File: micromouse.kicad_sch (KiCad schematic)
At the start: 12 parts, among them SW1 SW_SPST, SW2 SW_Push, U1 BUCK, U2 STM32 Blackpill, U3 N20 encoder right, U4 N20 encoder left, U5 TB6612FNG, U6 VL53L0X left, U7 VL53L0X right, U8 VL53L0X middle

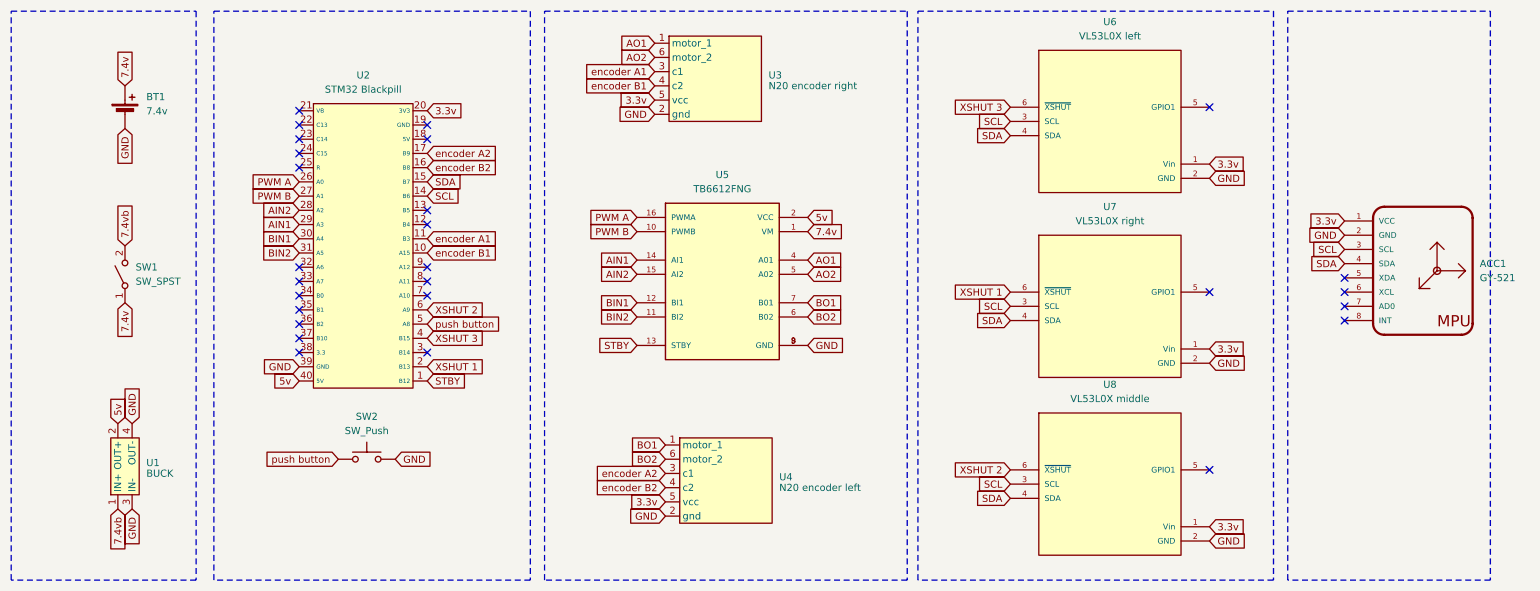
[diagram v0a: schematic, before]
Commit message: schematic and footprint changes
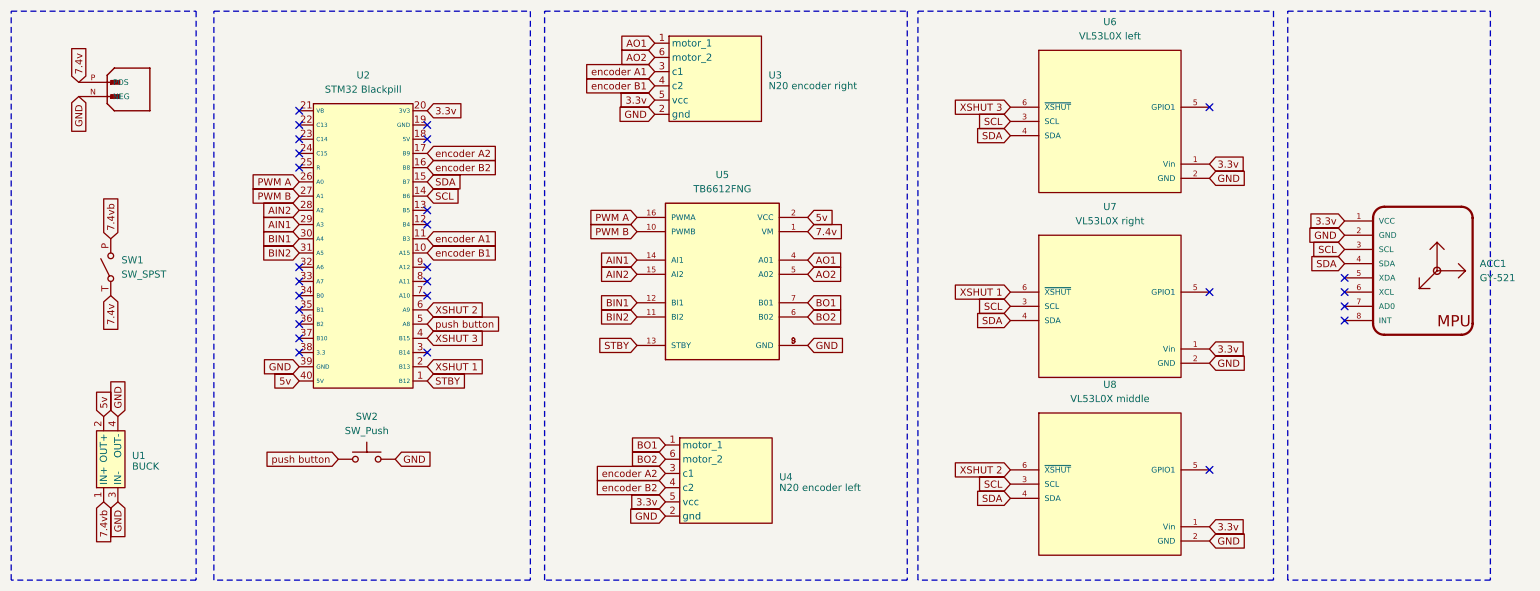
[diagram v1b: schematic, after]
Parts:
- removed BT1: 7.4v, symbol Device:Battery_Cell
- removed U5: TB6612FNG, TB6612FNG:TB6612FNG, symbol tb6612fng:ROB-14450
- added J1: XT60-M, XT60:AMASS_XT60-M, symbol XT60-M:XT60-M
- added U5: TB6612FNG, TB6612FNG:TB6612FNG, symbol TB66:TB6612FNG
- U3, U4: footprint Connector_PinHeader_2.00mm:PinHeader_1x06_P2.00mm_Vertical -> Connector_PinHeader_2.54mm:PinHeader_1x06_P2.54mm_Vertical
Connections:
- net 5v: now also U5.2 (VCC)
- net 7.4v: now also SW1.T (A), J1.P (POS), U5.1 (VM); no longer SW1.1 (A)
- net 7.4vb: now also SW1.P (B); no longer SW1.2 (B)
- net AIN1: now also U5.14 (AI1)
- net AIN2: now also U5.15 (AI2)
- net AO1 : now also U5.4 (A01)
- net AO2: now also U5.5 (A02)
- net BIN1: now also U5.12 (BI1)
- net BIN2: now also U5.11 (BI2)
- net BO1: now also U5.7 (B01)
- net BO2: now also U5.6 (B02)
- net GND: now also J1.N (NEG), U5.3 (GND), U5.8 (GND), U5.9 (GND)
- net PWM A: now also U5.16 (PWMA)
- net PWM B: now also U5.10 (PWMB)
- net STBY: now also U5.13 (STBY)
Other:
- moved on the sheet: SW1, U1

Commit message: routing
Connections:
- net AO1  is gone; now on net AO1: U5.4 (A01)
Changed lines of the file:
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@@
 		)
 	)
-	(global_label "AO1 "
+	(global_label "AO1"
 		(shape input)
 		(at 158.115 84.455 0)
@@
 		)
 		(property "Intersheetrefs" "${INTERSHEET_REFS}"
-			(at 165.6964 84.455 0)
+			(at 164.7288 84.455 0)
 			(effects
 				(font

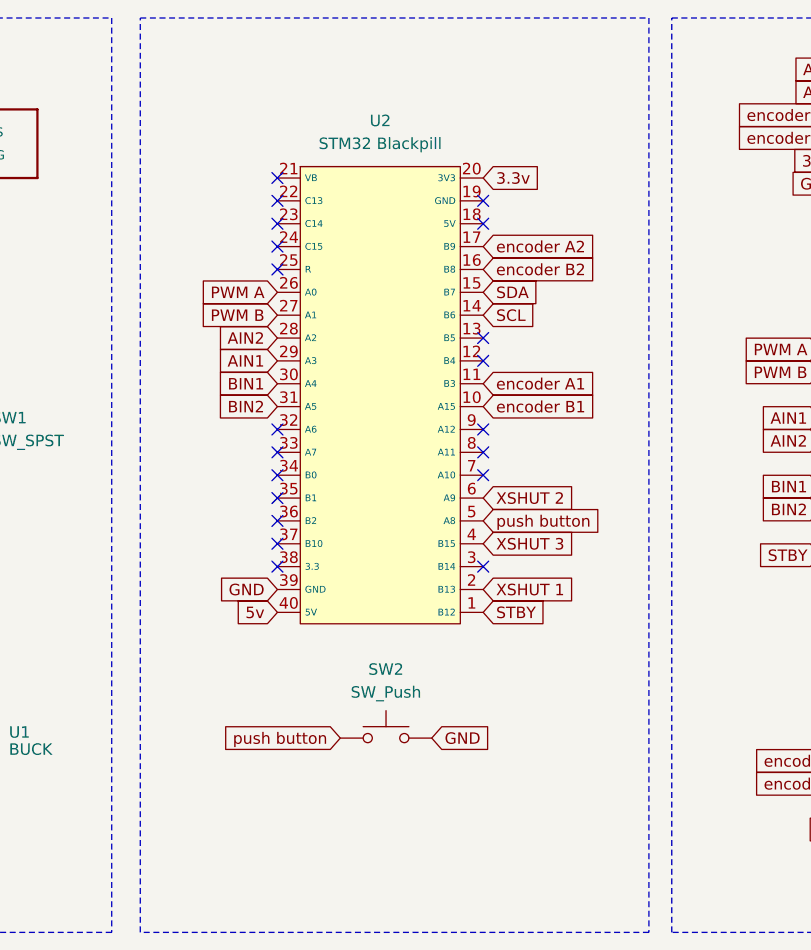
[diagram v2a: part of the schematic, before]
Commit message: ll
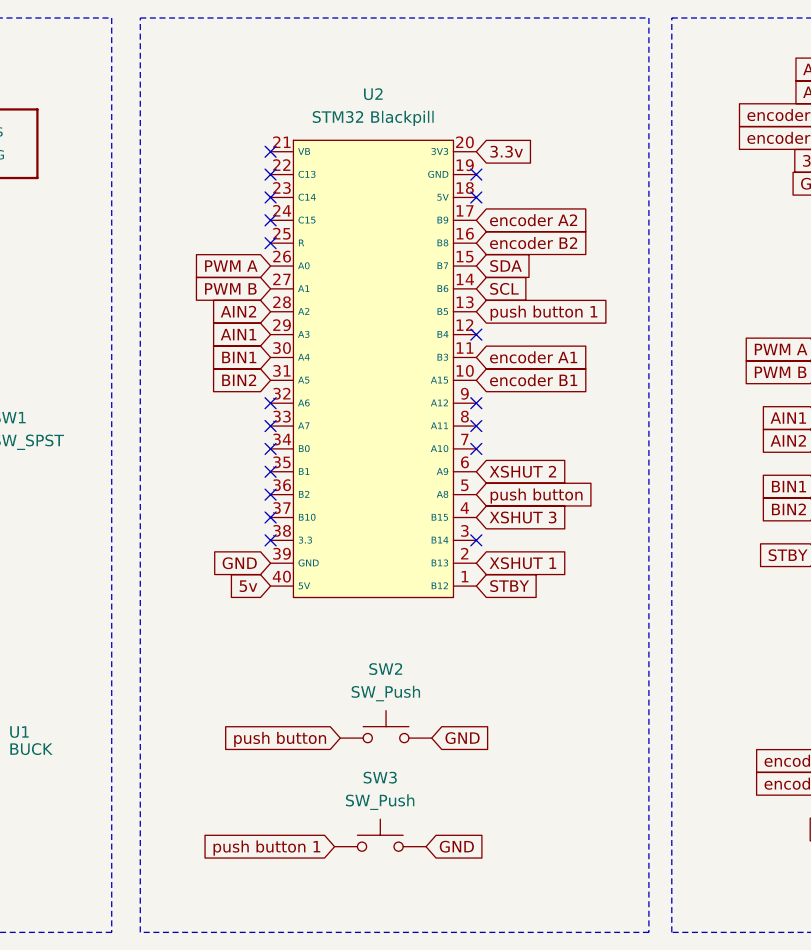
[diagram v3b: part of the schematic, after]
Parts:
- added SW3: SW_Push, push button:push_button, symbol Switch:SW_Push
- U5: footprint TB6612FNG:TB6612FNG -> Tb6612fng:TB6612FNG
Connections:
- net GND: now also SW3.2
- net push button 1: now reaches U2.13 (B5)
- net push button 1: now also SW3.1
- no-connect marks 27 -> 26
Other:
- moved on the sheet: U2

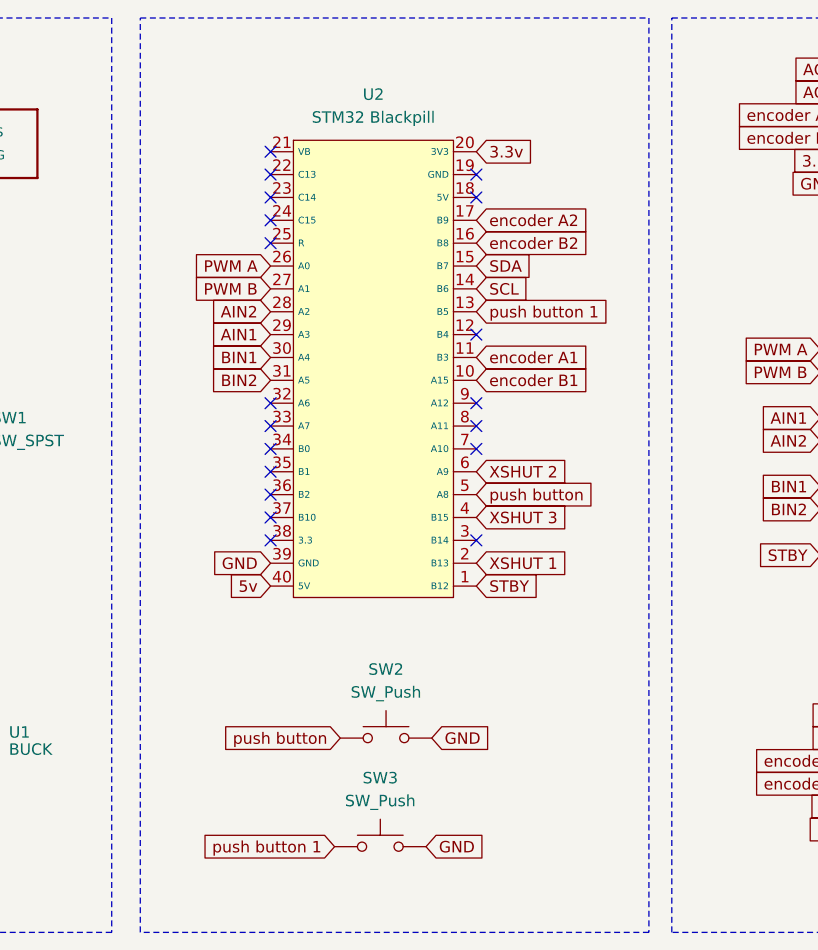
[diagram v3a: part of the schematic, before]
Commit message: pcb changes
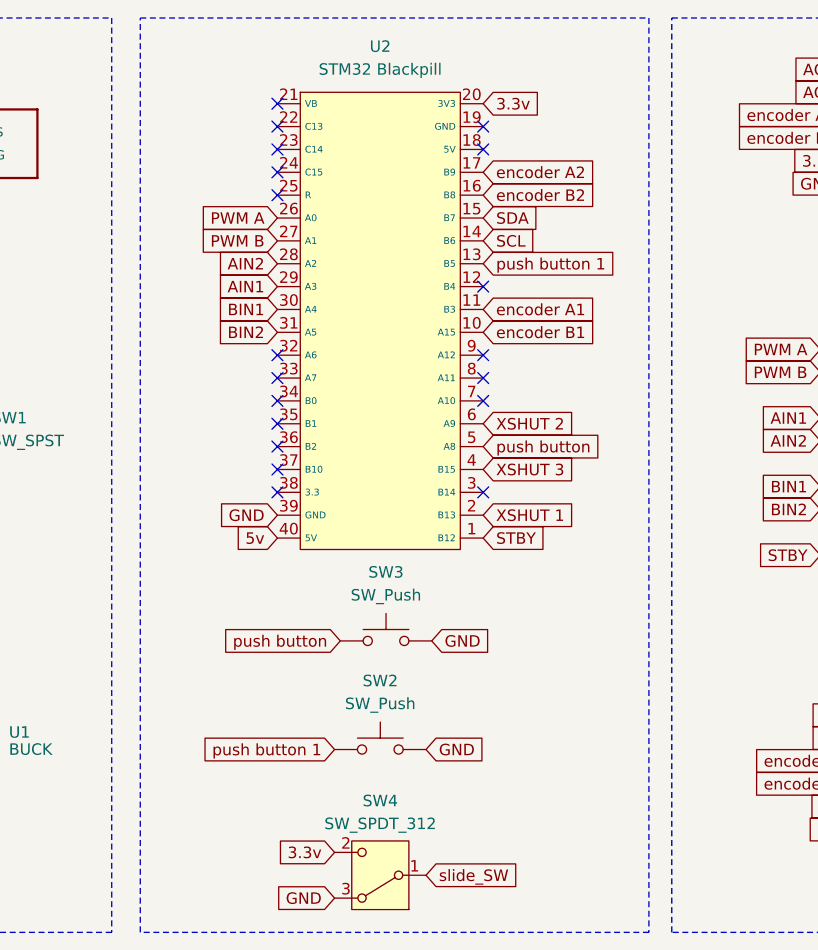
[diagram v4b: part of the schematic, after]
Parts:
- added SW4: SW_SPDT_312, slide switch:SLIDE SW, symbol Switch:SW_SPDT_312
- U5: footprint Tb6612fng:TB6612FNG -> TB6612FNG:TB6612FNG
- renumbered SW3 to SW2, SW2 to SW3
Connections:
- net 3.3v: now also SW4.2 (C)
- net GND: now also SW4.3 (A)
- new net slide_SW: SW4.1 (B)
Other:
- moved on the sheet: SW2, SW3, U2
